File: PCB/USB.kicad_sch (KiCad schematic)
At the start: 1 part, among them J2 USB_C_Receptacle_USB2.0_16P

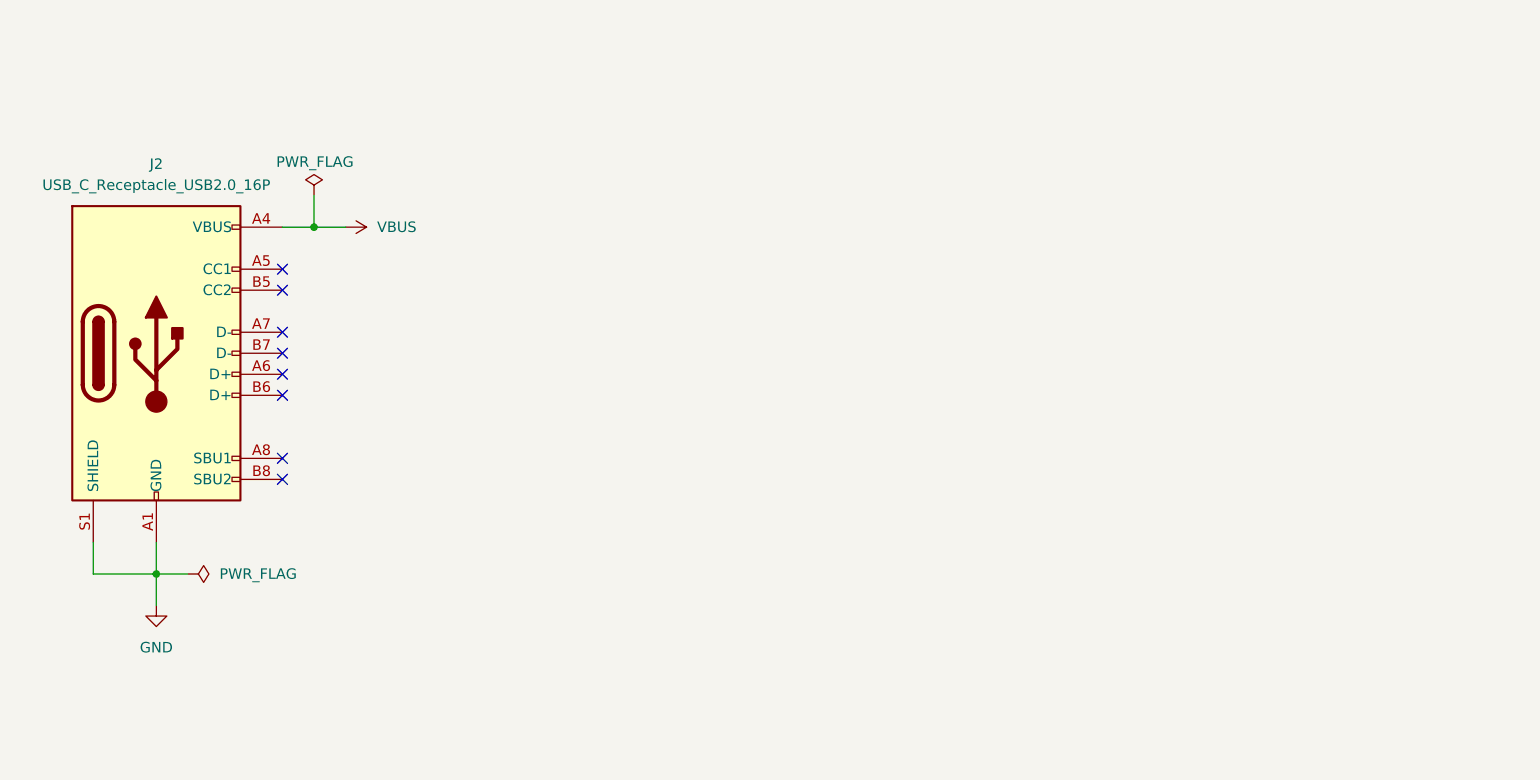
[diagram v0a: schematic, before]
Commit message: Finished the schematic.
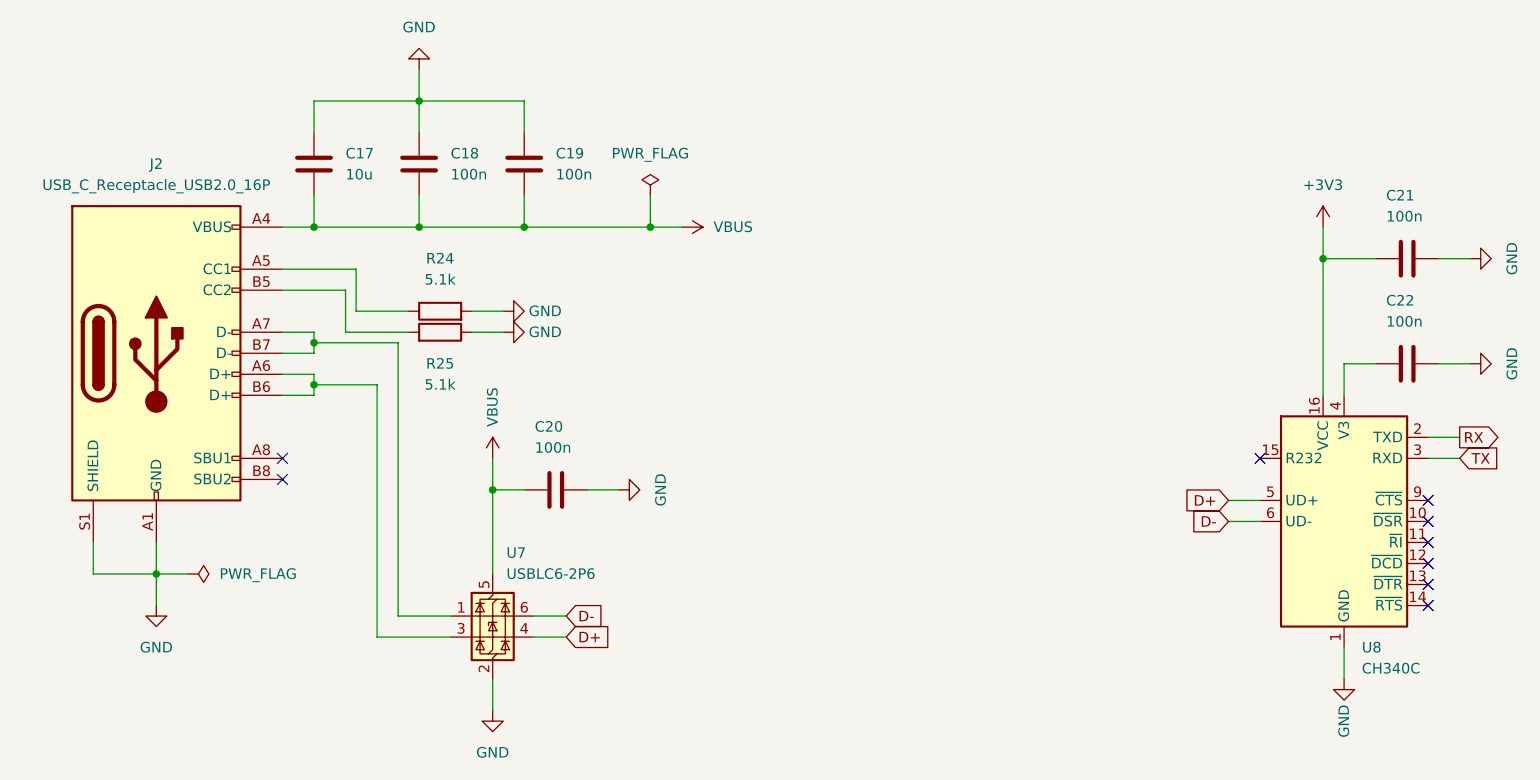
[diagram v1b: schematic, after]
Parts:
- added C17: 10u, Capacitor_SMD:C_0201_0603Metric, symbol Device:C
- added C18, C19, C20, C21, C22: 100n, Capacitor_SMD:C_0201_0603Metric, symbol Device:C
- added R24, R25: 5.1k, Resistor_SMD:R_0201_0603Metric, symbol Device:R
- added U7: USBLC6-2P6, Package_TO_SOT_SMD:SOT-666, symbol Power_Protection:USBLC6-2P6
- added U8: CH340C, Package_SO:SOIC-16_3.9x9.9mm_P1.27mm, symbol Interface_USB:CH340C
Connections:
- net GND: now also C17.1, C18.1, C19.1, C20.2, C21.2, C22.2, R24.2, R25.1, U7.2 (GND), U8.1 (GND)
- net VBUS: now also C17.2, C18.2, C19.2, C20.1, U7.5 (VBUS)
- net at J2.A5 (CC1): now also R24.1
- net at J2.A6 (D+): now also J2.B6 (D+), U7.3 (I/O2)
- net at J2.A7 (D-): now also J2.B7 (D-), U7.1 (I/O1)
- net at J2.B5 (CC2): now also R25.2
- new net: C22.1, U8.4 (V3)
- new net +3V3: C21.1, U8.16 (VCC)
- new net D+: U7.4 (I/O2), U8.5 (UD+)
- new net D-: U7.6 (I/O1), U8.6 (UD-)
- new net RX: U8.2 (TXD)
- new net TX: U8.3 (RXD)
- no-connect marks 8 -> 9
